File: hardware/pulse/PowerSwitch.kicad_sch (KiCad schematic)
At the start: 22 parts, among them J1801 WAGO-2065, J1802 WAGO-2065, U1801 BTT6010

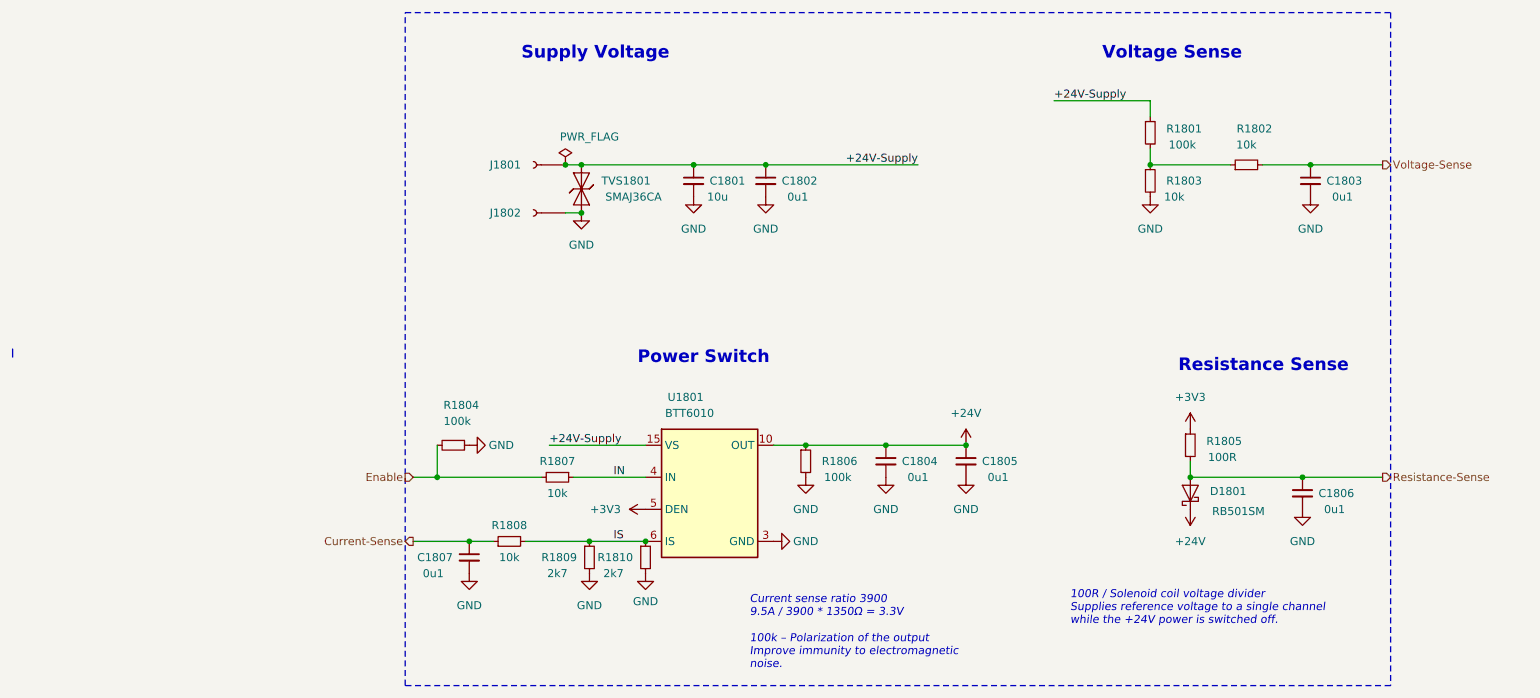
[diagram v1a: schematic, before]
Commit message: Update parts
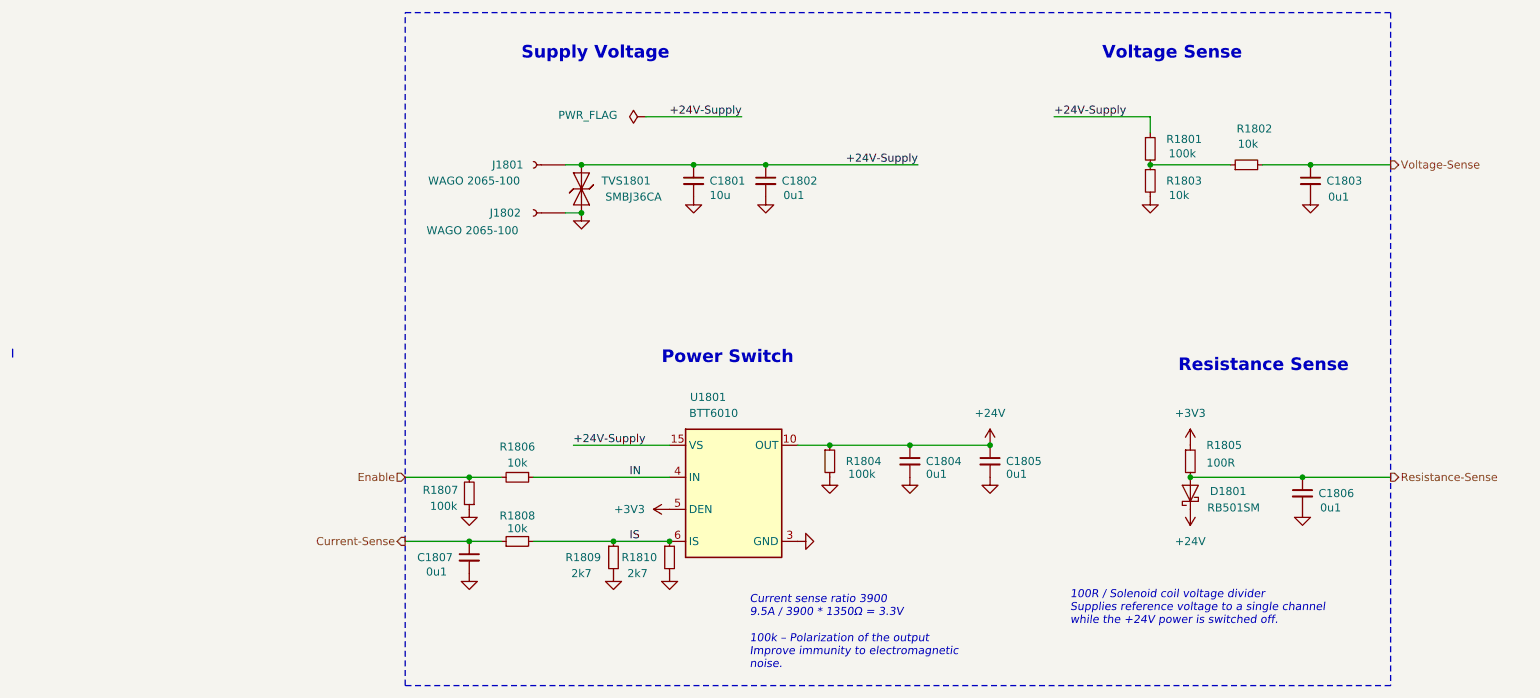
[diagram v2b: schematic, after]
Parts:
- C1801: footprint Capacitor_SMD:C_1210_3225Metric -> V2_Capacitor_SMD:C_1210; symbol Device:C_Small -> V2_Device:C_1210_10u; Manufacturer (none) -> TDK; Mouser (none) -> 810-CNA6P1X7R1H106K2; Product (none) -> CNA6P1X7R1H106K250AE; Rating (none) -> 50V; Voltage (none) -> 50V
- C1802, C1803, C1804, C1805, C1806, C1807: footprint Capacitor_SMD:C_0603_1608Metric -> V2_Capacitor_SMD:C_0603; symbol Device:C_Small -> V2_Device:C_0603_0u1; Manufacturer (none) -> TDK; Mouser (none) -> 810-CGA3E2X7R1H104MA; Product (none) -> CGA3E2X7R1H104M080AA
- D1801: footprint Diode_SMD:D_SOD-523 -> V2_Diode_SMD:D_SOD-523; Manufacturer (none) -> ROHM Semiconductor; Mouser (none) -> 755-RB501SM-30FHT2R; Product (none) -> RB501SM-30FHT2R
- J1801, J1802: value WAGO-2065 -> WAGO 2065-100; Manufacturer (none) -> WAGO; Product (none) -> 2065-100/998-403
- R1801: footprint Resistor_SMD:R_0603_1608Metric -> V2_Resistor_SMD:R_0603; symbol Device:R_Small -> V2_Device:R_0603_100k; Manufacturer (none) -> Vishay; Mouser (none) -> 71-CRCW0603100KFKEAC; Product (none) -> CRCW0603100KFKEAC; Rating (none) -> 100mW
- R1802, R1803, R1808: footprint Resistor_SMD:R_0603_1608Metric -> V2_Resistor_SMD:R_0603; symbol Device:R_Small -> V2_Device:R_0603_10k; Manufacturer (none) -> Vishay; Mouser (none) -> 71-CRCW060310K0FKEAC; Product (none) -> CRCW060310K0FKEAC; Rating (none) -> 100mW
- R1804: renamed from R1806; footprint Resistor_SMD:R_0603_1608Metric -> V2_Resistor_SMD:R_0603; symbol Device:R_Small -> V2_Device:R_0603_100k; Manufacturer (none) -> Vishay; Mouser (none) -> 71-CRCW0603100KFKEAC; Product (none) -> CRCW0603100KFKEAC; Rating (none) -> 100mW
- R1805: footprint Resistor_SMD:R_0603_1608Metric -> V2_Resistor_SMD:R_0603; symbol Device:R_Small -> V2_Device:R_0603_100R; Manufacturer (none) -> Vishay; Mouser (none) -> 71-CRCW0603100RFKEAH; Product (none) -> CRCW0603100RFKEAHP; Rating (none) -> 330mW
- R1806: renamed from R1807; footprint Resistor_SMD:R_0603_1608Metric -> V2_Resistor_SMD:R_0603; symbol Device:R_Small -> V2_Device:R_0603_10k; Manufacturer (none) -> Vishay; Mouser (none) -> 71-CRCW060310K0FKEAC; Product (none) -> CRCW060310K0FKEAC; Rating (none) -> 100mW
- R1807: renamed from R1804; footprint Resistor_SMD:R_0603_1608Metric -> V2_Resistor_SMD:R_0603; symbol Device:R_Small -> V2_Device:R_0603_100k; Manufacturer (none) -> Vishay; Mouser (none) -> 71-CRCW0603100KFKEAC; Product (none) -> CRCW0603100KFKEAC; Rating (none) -> 100mW
- R1809, R1810: footprint Resistor_SMD:R_0603_1608Metric -> V2_Resistor_SMD:R_0603; symbol Device:R_Small -> V2_Device:R_0603_2k7; Manufacturer (none) -> Vishay; Mouser (none) -> 71-CRCW06032K70FKEAC; Product (none) -> CRCW06032K70FKEAC; Rating (none) -> 100mW
- TVS1801: value SMAJ36CA -> SMBJ36CA; footprint Diode_SMD:D_SMA -> V2_Diode_SMD:D_SMB; symbol V2_Diode:SMAJ36CA -> V2_Diode:SMBJ36CA; Manufacturer (none) -> Bourns; Mouser (none) -> 652-SMBJ36CA-Q; Product (none) -> SMBJ36CA-Q; Rating (none) -> 36V
- U1801: Manufacturer (none) -> Infineon; Mouser (none) -> 726-BTT60101ERBXUMA1; Product (none) -> BTT60101ERBXUMA1
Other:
- moved on the sheet: C1804, C1805, R1801, R1804, R1805, R1806, R1807, R1808, R1809, R1810, U1801

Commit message: Refresh
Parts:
- C1801: Rating 50V -> (none)
